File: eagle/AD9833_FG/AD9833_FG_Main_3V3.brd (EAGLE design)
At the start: 53 x 63.5 mm, 19 parts, among them IC1 ATMEGA48/88/168, IC2 AD9833_MODULE, IC3 TA48M033F

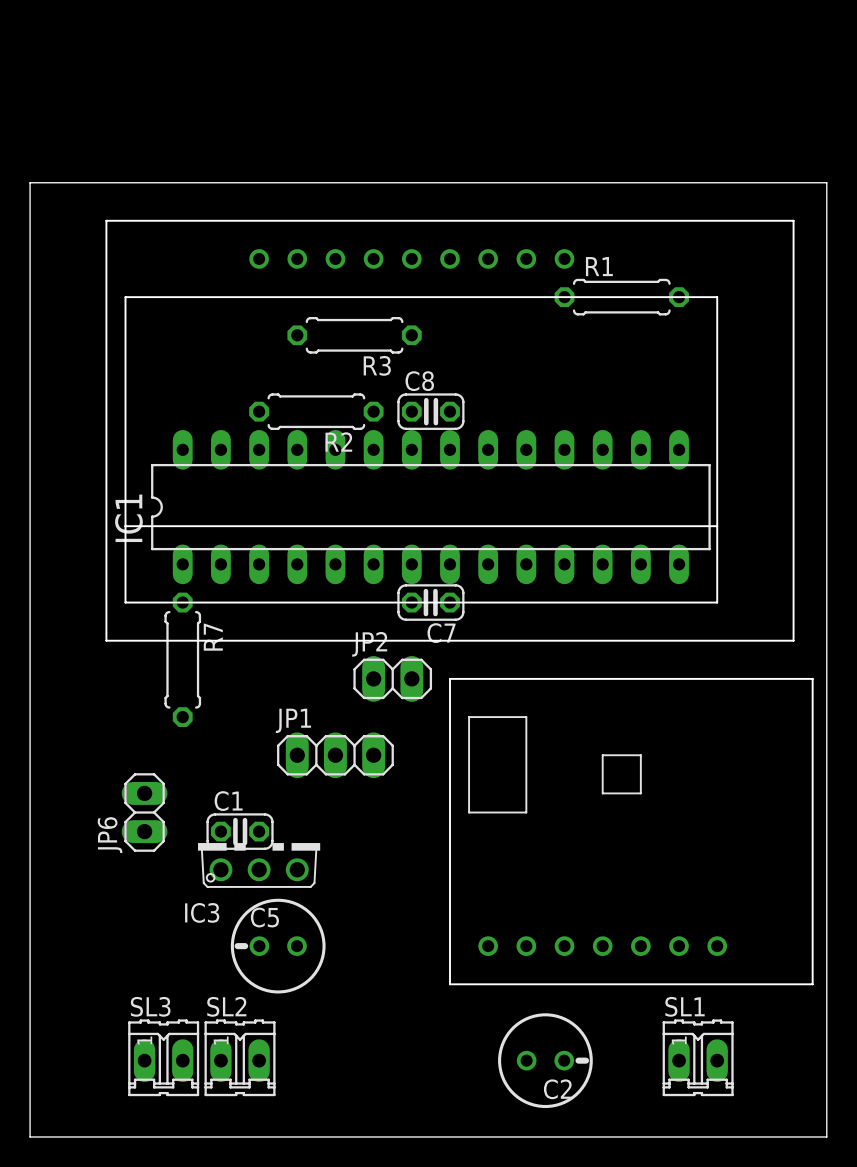
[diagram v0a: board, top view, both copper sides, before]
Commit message: Update eagle files
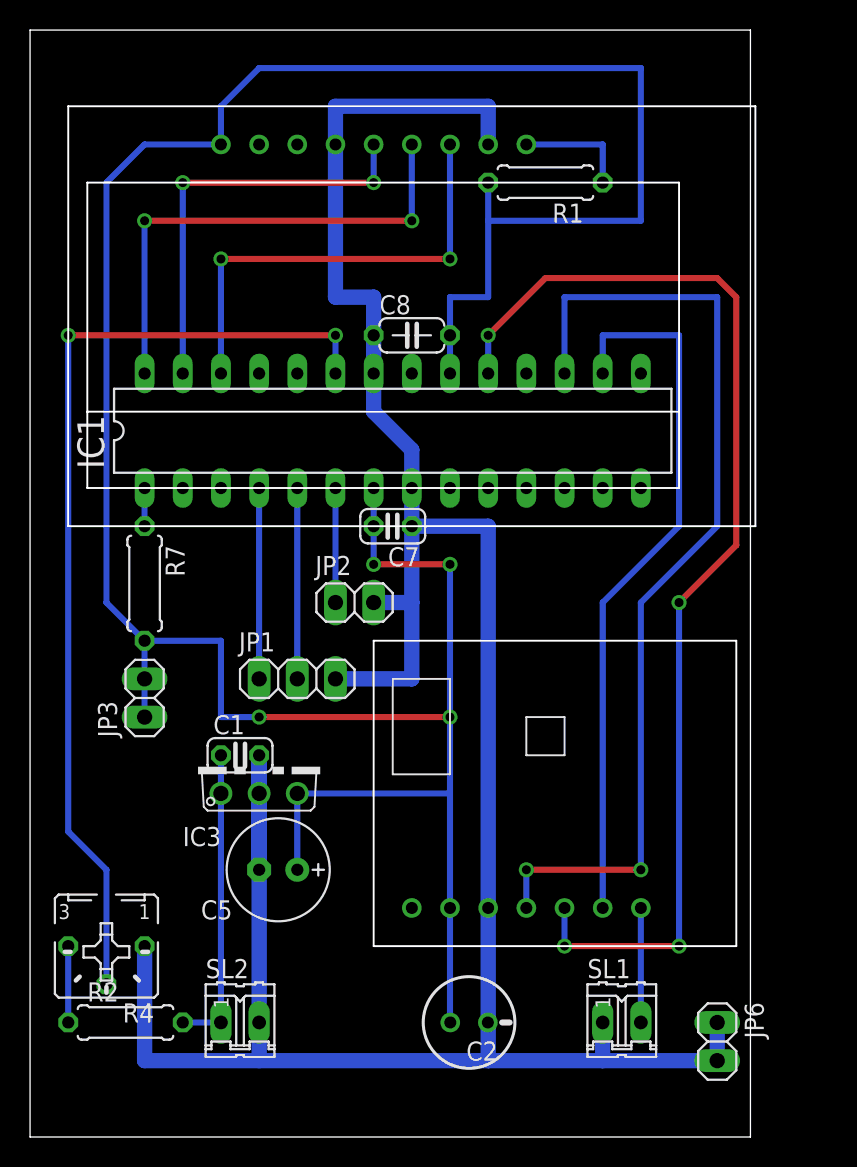
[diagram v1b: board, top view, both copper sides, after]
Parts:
- removed R3: 3.3k, rcl:0207/7
- removed SL3: PWR, con-amp-quick:02P
- added JP3: TP_3V3, pinhead:1X02
- added R4: 100k, pot:B25P
- C5: device rcl:SANYO-OSCON_C -> rcl:E2,5-7
- C8: device rcl:C025-024X044 -> rcl:C050-024X044
- R2: value 12k -> 220k
- moved R2 42.6 mm to (6.35, 7.62), turned to 0 degrees
- moved JP6 41.0 mm to (45.7, 6.35), turned to 270 degrees
- moved R1 9.16 mm to (34.3, 63.5), turned to 180 degrees
- moved LCD1 8.03 mm to (21.6, 61.0)
- moved SL1 5.68 mm to (39.4, 7.62)
- moved IC1 5.68 mm to (22.9, 47.0)
- moved JP1 5.68 mm to (17.8, 30.5)
- moved JP2 5.68 mm to (21.6, 35.6)
- moved C7 5.68 mm to (24.1, 40.6)
- moved IC2 5.68 mm to (35.6, 17.8)
- moved C2 5.68 mm to (29.2, 7.62)
- moved R7 5.68 mm to (7.62, 36.8)
- moved C8 5.24 mm to (25.4, 53.3)
- moved C5 5.08 mm to (16.5, 17.8), turned to 180 degrees
- moved C1 5.08 mm to (14.0, 25.4)
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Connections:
- new net N$11: R2.1, R4.E
- net +3V3: now also JP3.1, JP3.2
- net GND: now also R4.A; no longer R3.1, SL3.1
- net N$15: no longer SL3.2
- net N$16: now also R4.S; no longer R2.1, R3.2
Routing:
- net +3V3: track 0.00 -> 193.7 mm, vias 0 -> 4
- net GND: track 0.00 -> 181.4 mm
- net N$2: track 0.00 -> 76.1 mm, vias 0 -> 4
- net N$1: track 0.00 -> 65.6 mm, vias 0 -> 2
- net N$16: track 0.00 -> 64.6 mm, vias 0 -> 2
- net N$3: track 0.00 -> 47.8 mm
- net N$4: track 0.00 -> 33.0 mm, vias 0 -> 2
- net N$7: track 0.00 -> 30.5 mm, vias 0 -> 2
- net N$5: track 0.00 -> 27.9 mm, vias 0 -> 2
- net N$15: track 0.00 -> 20.3 mm
- net N$9: track 0.00 -> 12.7 mm
- net N$8: track 0.00 -> 12.7 mm
- net N$14: track 0.00 -> 7.62 mm
- net N$6: track 0.00 -> 7.62 mm
- net N$10: track 0.00 -> 7.62 mm
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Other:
- board size 53 x 63.5 mm -> 47.9 x 73.7 mm
